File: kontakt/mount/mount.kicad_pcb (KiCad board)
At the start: 2 copper layers, 60.6 x 111.8 mm, 28 parts, among them J1 INPUT, J10 USB_B, J11 INPUT, J12 INPUT, J13 INPUT, J14 INPUT, J15 Conn_01x15_Male, J16 Conn_01x04_Male, J2 INPUT, J3 INPUT, J4 INPUT, J5 INPUT, J6 INPUT, J7 INPUT, J8 INPUT, J9 INPUT

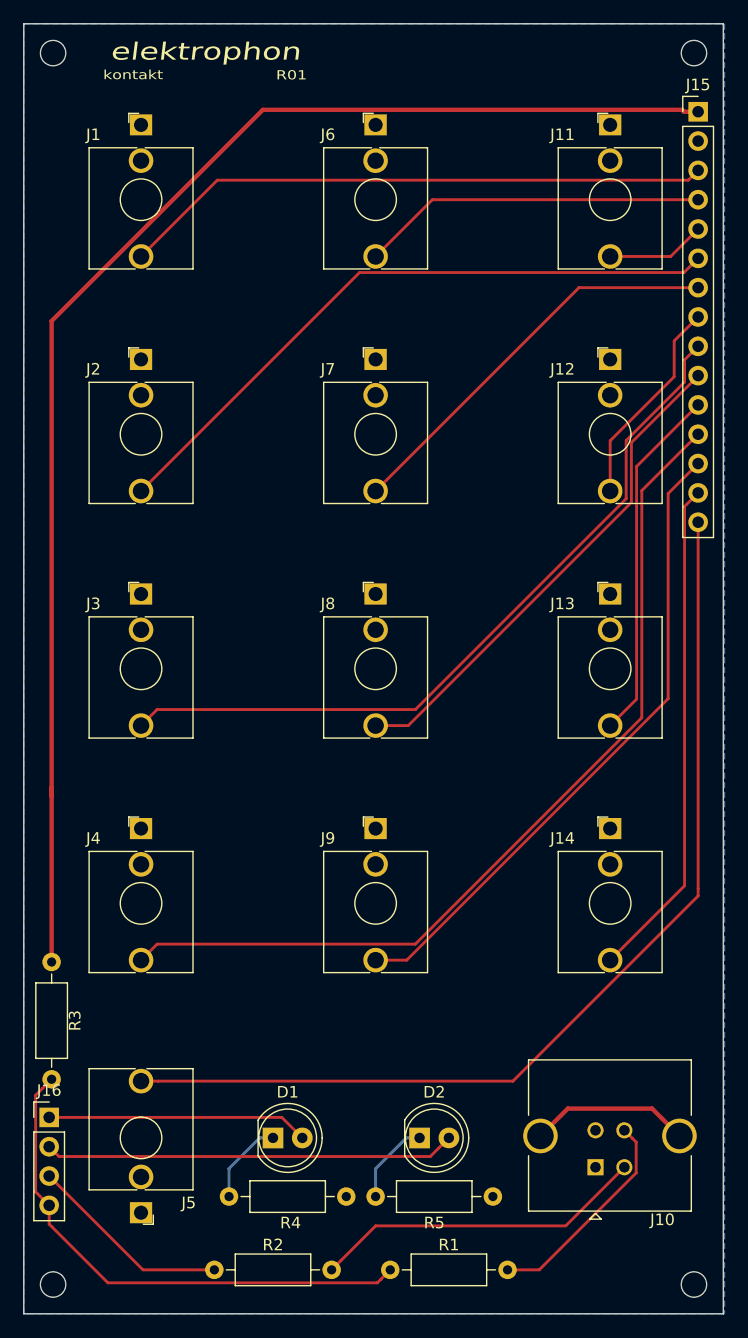
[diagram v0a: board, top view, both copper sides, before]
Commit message: update kontakt
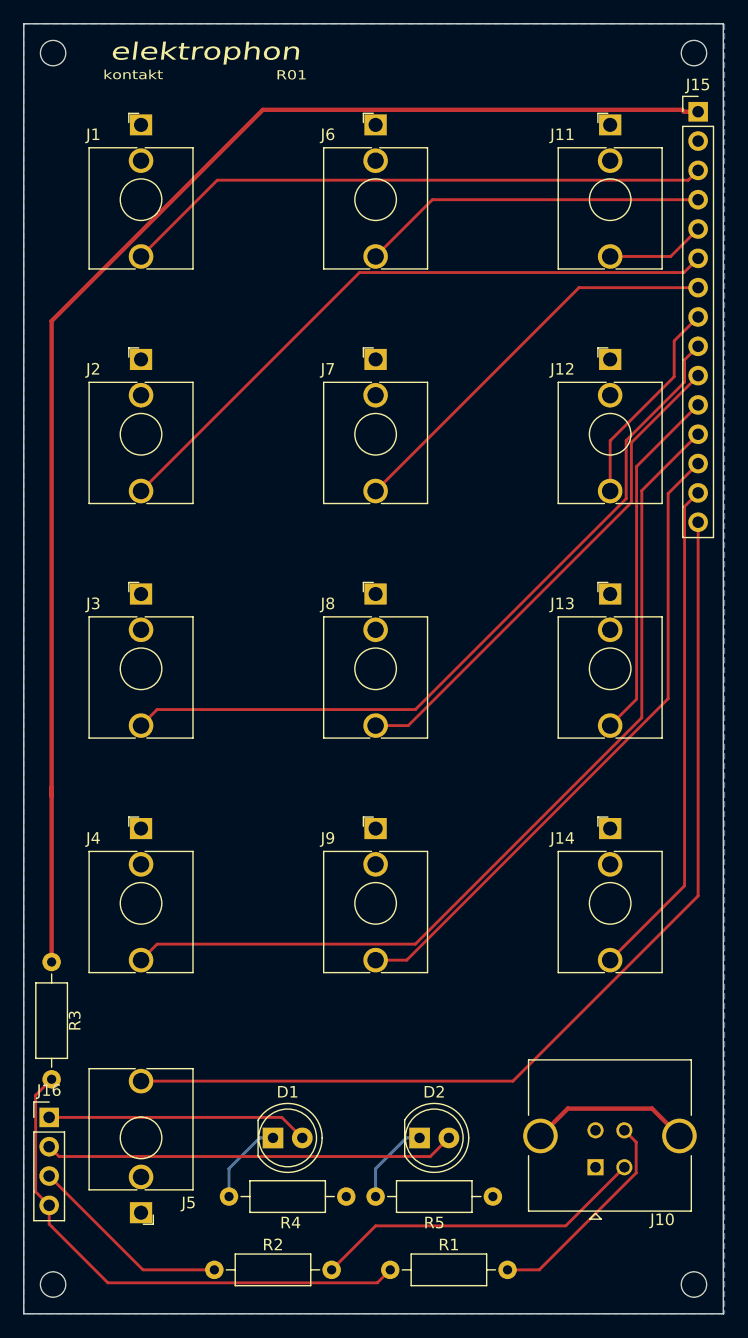
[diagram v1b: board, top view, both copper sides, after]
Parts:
- R3: value 20 -> 1k5
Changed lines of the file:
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@@
     (thickness 1.6)
     (drawings 4)
-    (tracks 92)
+    (tracks 84)
     (zones 0)
     (modules 28)
@@
       (effects (font (size 1 1) (thickness 0.15)))
     )
-    (fp_text value 20 (at 5.08 2.37 90) (layer F.Fab)
+    (fp_text value 1k5 (at 5.08 2.37 90) (layer F.Fab)
       (effects (font (size 1 1) (thickness 0.15)))
     )
@@
   (segment (start 71.511359 58.254499) (end 53.213 76.552858) (width 0.381) (layer F.Cu) (net 1))
   (segment (start 107.823499 58.254499) (end 71.511359 58.254499) (width 0.381) (layer F.Cu) (net 1))
-  (segment (start 109.22 58.42) (end 107.989 58.42) (width 0.381) (layer F.Cu) (net 1))
+  (segment (start 109.22 58.42) (end 107.989 58.42) (width 0.381) (layer F.Cu) (net 1) (status 10))
   (segment (start 107.989 58.42) (end 107.823499 58.254499) (width 0.381) (layer F.Cu) (net 1))
-  (segment (start 53.213 116.967) (end 53.213 132.08) (width 0.381) (layer F.Cu) (net 1))
+  (segment (start 53.213 116.967) (end 53.213 132.08) (width 0.381) (layer F.Cu) (net 1) (status 20))
   (segment (start 53.213 76.552858) (end 53.213 116.967) (width 0.381) (layer F.Cu) (net 1))
   (segment (start 53.213 116.967) (end 53.213 117.729) (width 0.381) (layer F.Cu) (net 1))
-  (segment (start 71.24 147.32) (end 72.39 147.32) (width 0.25) (layer B.Cu) (net 3))
+  (segment (start 71.24 147.32) (end 72.39 147.32) (width 0.25) (layer B.Cu) (net 3) (status 20))
   (segment (start 68.58 149.98) (end 71.24 147.32) (width 0.25) (layer B.Cu) (net 3))
-  (segment (start 68.58 152.4) (end 68.58 149.98) (width 0.25) (layer B.Cu) (net 3))
-  (segment (start 83.94 147.32) (end 85.09 147.32) (width 0.25) (layer B.Cu) (net 4))
+  (segment (start 68.58 152.4) (end 68.58 149.98) (width 0.25) (layer B.Cu) (net 3) (status 10))
+  (segment (start 83.94 147.32) (end 85.09 147.32) (width 0.25) (layer B.Cu) (net 4) (status 20))
   (segment (start 81.28 149.98) (end 83.94 147.32) (width 0.25) (layer B.Cu) (net 4))
-  (segment (start 81.28 152.4) (end 81.28 149.98) (width 0.25) (layer B.Cu) (net 4))
-  (segment (start 73.152 145.542) (end 74.93 147.32) (width 0.25) (layer F.Cu) (net 5))
-  (segment (start 53 145.542) (end 73.152 145.542) (width 0.25) (layer F.Cu) (net 5))
-  (segment (start 86.730001 148.219999) (end 87.63 147.32) (width 0.25) (layer F.Cu) (net 6))
-  (segment (start 86.018001 148.931999) (end 86.730001 148.219999) (width 0.25) (layer F.Cu) (net 6))
+  (segment (start 81.28 152.4) (end 81.28 149.98) (width 0.25) (layer B.Cu) (net 4) (status 10))
+  (segment (start 73.152 145.542) (end 74.93 147.32) (width 0.25) (layer F.Cu) (net 5) (status 20))
+  (segment (start 53 145.542) (end 73.152 145.542) (width 0.25) (layer F.Cu) (net 5) (status 10))
+  (segment (start 86.018001 148.931999) (end 87.63 147.32) (width 0.25) (layer F.Cu) (net 6) (status 20))
   (segment (start 53.849999 148.931999) (end 86.018001 148.931999) (width 0.25) (layer F.Cu) (net 6))
-  (segment (start 53 148.082) (end 53.849999 148.931999) (width 0.25) (layer F.Cu) (net 6))
+  (segment (start 53 148.082) (end 53.849999 148.931999) (width 0.25) (layer F.Cu) (net 6) (status 10))
   (segment (start 67.570001 64.349999) (end 60.96 70.96) (width 0.25) (layer F.Cu) (net 7) (status 20))
   (segment (start 108.370001 64.349999) (end 67.570001 64.349999) (width 0.25) (layer F.Cu) (net 7))
@@
   (segment (start 109.22 86.36) (end 104.340034 91.239966) (width 0.25) (layer F.Cu) (net 10) (status 10))
   (segment (start 104.340034 91.239966) (end 104.340034 110.917168) (width 0.25) (layer F.Cu) (net 10))
-  (segment (start 62.466137 142.4) (end 60.96 142.4) (width 0.25) (layer F.Cu) (net 11))
-  (segment (start 93.177202 142.4) (end 62.466137 142.4) (width 0.25) (layer F.Cu) (net 11))
+  (segment (start 93.177202 142.4) (end 60.96 142.4) (width 0.25) (layer F.Cu) (net 11) (status 20))
   (segment (start 109.22 126.357202) (end 93.177202 142.4) (width 0.25) (layer F.Cu) (net 11))
-  (segment (start 109.22 125.73) (end 109.22 126.357202) (width 0.25) (layer F.Cu) (net 11))
-  (segment (start 109.22 93.98) (end 109.22 125.73) (width 0.25) (layer F.Cu) (net 11))
+  (segment (start 109.22 93.98) (end 109.22 126.357202) (width 0.25) (layer F.Cu) (net 11) (status 10))
   (segment (start 86.2 66.04) (end 81.28 70.96) (width 0.25) (layer F.Cu) (net 12) (status 20))
   (segment (start 109.22 66.04) (end 86.2 66.04) (width 0.25) (layer F.Cu) (net 12) (status 10))
@@
   (segment (start 106.622011 109.271602) (end 83.973613 131.92) (width 0.25) (layer F.Cu) (net 15))
   (segment (start 106.622011 91.497989) (end 106.622011 109.271602) (width 0.25) (layer F.Cu) (net 15))
-  (segment (start 103.529999 147.359999) (end 102.83 146.66) (width 0.25) (layer F.Cu) (net 16))
-  (segment (start 92.71 158.75) (end 95.457002 158.75) (width 0.25) (layer F.Cu) (net 16))
+  (segment (start 103.855001 147.685001) (end 102.83 146.66) (width 0.25) (layer F.Cu) (net 16) (status 20))
+  (segment (start 92.71 158.75) (end 95.457002 158.75) (width 0.25) (layer F.Cu) (net 16) (status 10))
   (segment (start 103.855001 150.352001) (end 103.855001 147.685001) (width 0.25) (layer F.Cu) (net 16))
   (segment (start 95.457002 158.75) (end 103.855001 150.352001) (width 0.25) (layer F.Cu) (net 16))
-  (segment (start 103.855001 147.685001) (end 103.529999 147.359999) (width 0.25) (layer F.Cu) (net 16))
-  (segment (start 81.28 154.94) (end 78.269999 157.950001) (width 0.25) (layer F.Cu) (net 17))
-  (segment (start 78.269999 157.950001) (end 77.47 158.75) (width 0.25) (layer F.Cu) (net 17))
+  (segment (start 81.28 154.94) (end 77.47 158.75) (width 0.25) (layer F.Cu) (net 17) (status 20))
   (segment (start 97.75 154.94) (end 81.28 154.94) (width 0.25) (layer F.Cu) (net 17))
-  (segment (start 102.83 149.86) (end 97.75 154.94) (width 0.25) (layer F.Cu) (net 17))
+  (segment (start 102.83 149.86) (end 97.75 154.94) (width 0.25) (layer F.Cu) (net 17) (status 10))
   (segment (start 106.84 70.96) (end 101.6 70.96) (width 0.25) (layer F.Cu) (net 18) (status 20))
   (segment (start 109.22 68.58) (end 106.84 70.96) (width 0.25) (layer F.Cu) (net 18) (status 10))
@@
   (segment (start 101.6 131.92) (end 108.044999 125.475001) (width 0.25) (layer F.Cu) (net 21) (status 10))
   (segment (start 108.044999 125.475001) (end 108.044999 92.615001) (width 0.25) (layer F.Cu) (net 21))
-  (segment (start 61.128 158.75) (end 67.31 158.75) (width 0.25) (layer F.Cu) (net 22))
-  (segment (start 53 150.622) (end 61.128 158.75) (width 0.25) (layer F.Cu) (net 22))
-  (segment (start 81.750001 159.549999) (end 82.55 158.75) (width 0.25) (layer F.Cu) (net 23))
-  (segment (start 81.424999 159.875001) (end 81.750001 159.549999) (width 0.25) (layer F.Cu) (net 23))
+  (segment (start 61.128 158.75) (end 67.31 158.75) (width 0.25) (layer F.Cu) (net 22) (status 20))
+  (segment (start 53 150.622) (end 61.128 158.75) (width 0.25) (layer F.Cu) (net 22) (status 10))
+  (segment (start 81.424999 159.875001) (end 82.55 158.75) (width 0.25) (layer F.Cu) (net 23) (status 20))
   (segment (start 58.08892 159.875001) (end 81.424999 159.875001) (width 0.25) (layer F.Cu) (net 23))
   (segment (start 53.24696 155.03304) (end 53 154.78608) (width 0.25) (layer F.Cu) (net 23))
-  (segment (start 53 154.78608) (end 53 153.162) (width 0.25) (layer F.Cu) (net 23))
+  (segment (start 53 154.78608) (end 53 153.162) (width 0.25) (layer F.Cu) (net 23) (status 20))
   (segment (start 53.24696 155.03304) (end 58.08892 159.875001) (width 0.25) (layer F.Cu) (net 23))
-  (segment (start 52.413001 143.039999) (end 53.213 142.24) (width 0.25) (layer F.Cu) (net 23))
-  (segment (start 53 153.162) (end 51.824999 151.986999) (width 0.25) (layer F.Cu) (net 23))
-  (segment (start 51.824999 143.628001) (end 52.413001 143.039999) (width 0.25) (layer F.Cu) (net 23))
+  (segment (start 51.824999 143.628001) (end 53.213 142.24) (width 0.25) (layer F.Cu) (net 23) (status 20))
+  (segment (start 53 153.162) (end 51.824999 151.986999) (width 0.25) (layer F.Cu) (net 23) (status 10))
   (segment (start 51.824999 151.986999) (end 51.824999 143.628001) (width 0.25) (layer F.Cu) (net 23))
-  (segment (start 106.100001 145.650001) (end 107.6 147.15) (width 0.381) (layer F.Cu) (net 24))
-  (segment (start 105.23 144.78) (end 106.100001 145.650001) (width 0.381) (layer F.Cu) (net 24))
-  (segment (start 95.56 147.15) (end 97.93 144.78) (width 0.381) (layer F.Cu) (net 24))
+  (segment (start 105.23 144.78) (end 107.6 147.15) (width 0.381) (layer F.Cu) (net 24) (status 20))
+  (segment (start 95.56 147.15) (end 97.93 144.78) (width 0.381) (layer F.Cu) (net 24) (status 10))
   (segment (start 97.93 144.78) (end 105.23 144.78) (width 0.381) (layer F.Cu) (net 24))
   (zone (net 2) (net_name GND) (layer B.Cu) (hatch edge 0.508)
